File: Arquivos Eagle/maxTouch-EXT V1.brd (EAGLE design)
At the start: 35.6 x 53.3 mm, 11 parts

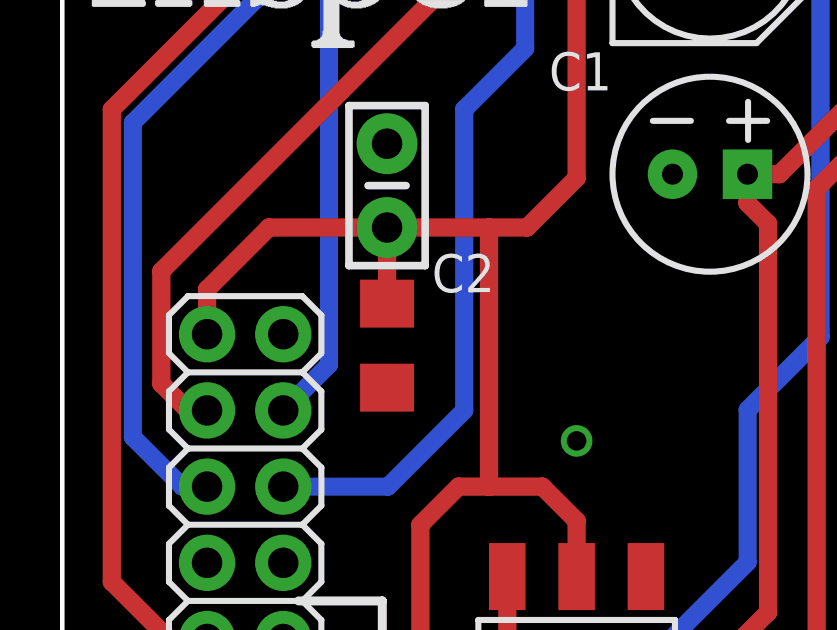
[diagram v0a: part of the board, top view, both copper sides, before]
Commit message: ~
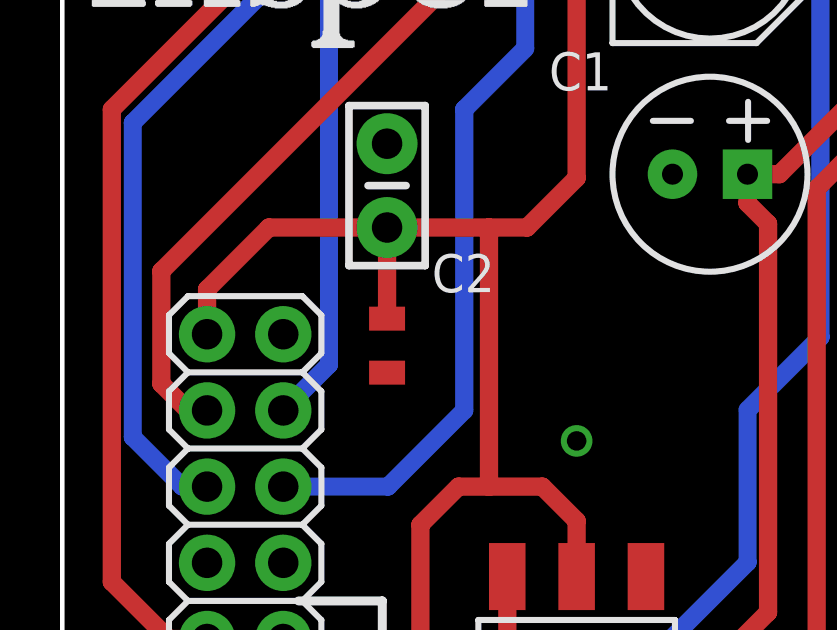
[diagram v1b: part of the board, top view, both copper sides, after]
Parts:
- C2: device SparkFun-Capacitors:1206 -> SparkFun-Capacitors:0805
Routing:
- net 3V3: track 65.5 -> 66.0 mm
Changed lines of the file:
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@@
 <attribute name="PROD_ID" value="CAP-12547" x="21.59" y="43.18" size="1.778" layer="27" display="off"/>
 </element>
-<element name="C2" library="SparkFun-Capacitors" package="1206" value="10uF" x="10.826" y="29.846" smashed="yes" rot="R270">
+<element name="C2" library="SparkFun-Capacitors" package="0805" value="10uF" x="10.826" y="29.846" smashed="yes" rot="R270">
 <attribute name="NAME" x="13.366" y="32.259" size="1.27" layer="21" font="vector" ratio="20" align="center"/>
 </element>
@@
 <wire x1="10.826" y1="33.783" x2="6.889" y2="33.783" width="0.6096" layer="1"/>
 <wire x1="6.889" y1="33.783" x2="4.826" y2="31.72" width="0.6096" layer="1"/>
-<wire x1="10.826" y1="31.246" x2="10.826" y2="33.783" width="0.6096" layer="1"/>
+<wire x1="10.826" y1="30.746" x2="10.826" y2="33.783" width="0.6096" layer="1"/>
 <contactref element="U1" pad="4"/>
 <contactref element="U1" pad="2"/>
